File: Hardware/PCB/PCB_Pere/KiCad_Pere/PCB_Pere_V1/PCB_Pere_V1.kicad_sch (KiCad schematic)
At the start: 23 parts, among them CN3 B4B-PH-K-S, U3 Buck LMR51625, U5 Buck LMR51625

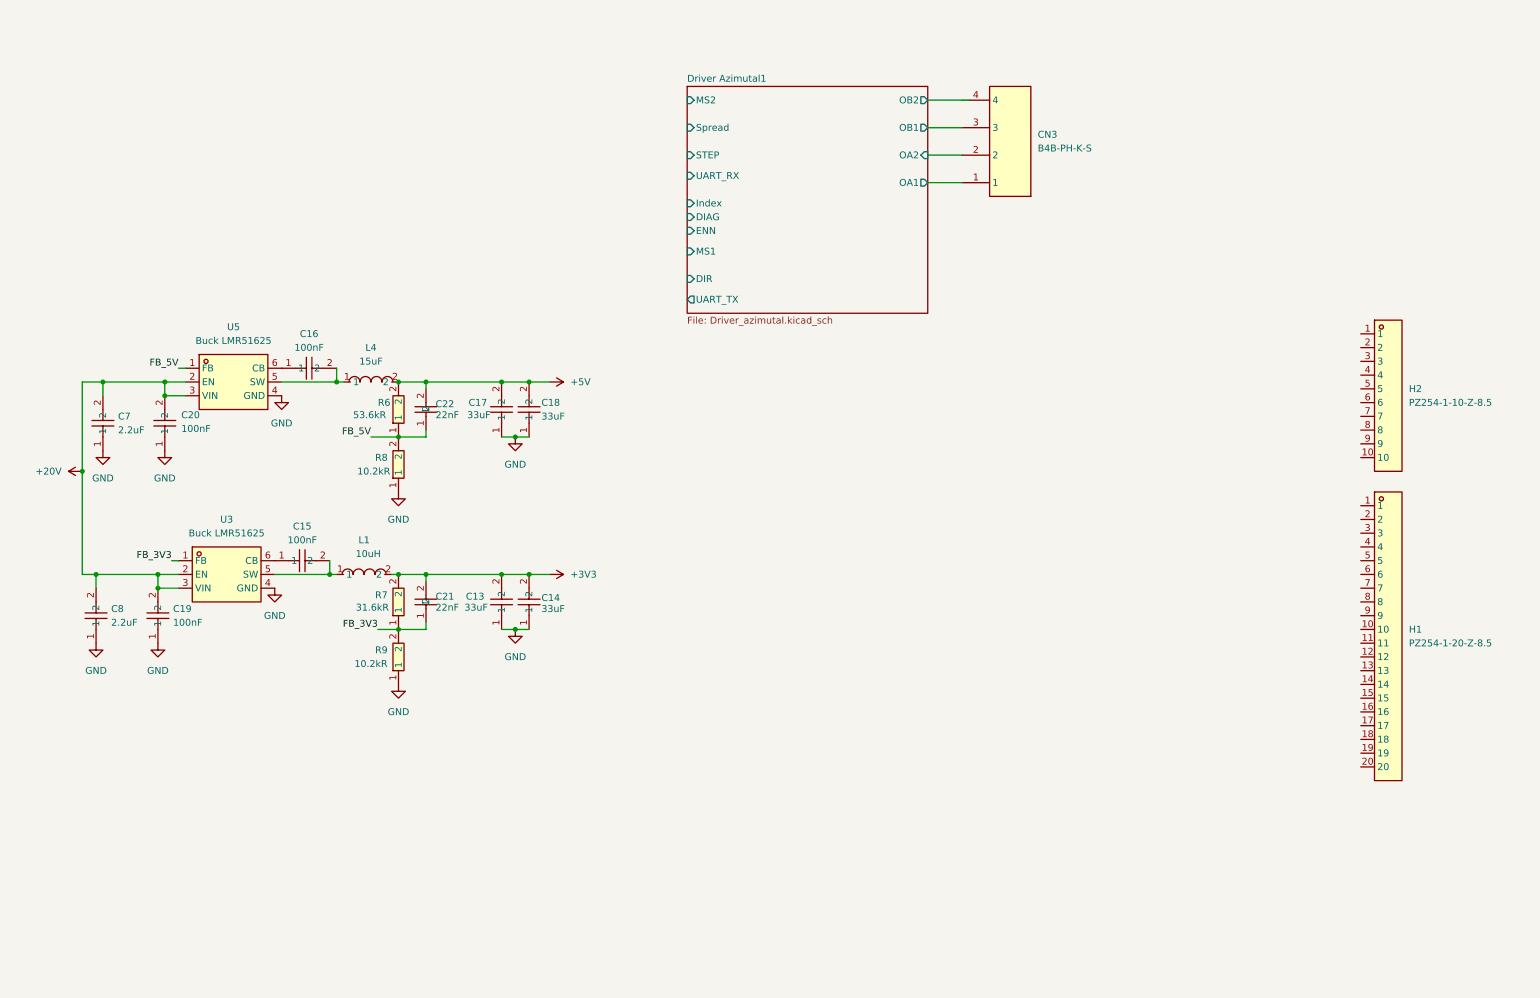
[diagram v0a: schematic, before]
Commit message: Routage toujours en attente oui je sais ça prend 10 000  ans mais it is what is
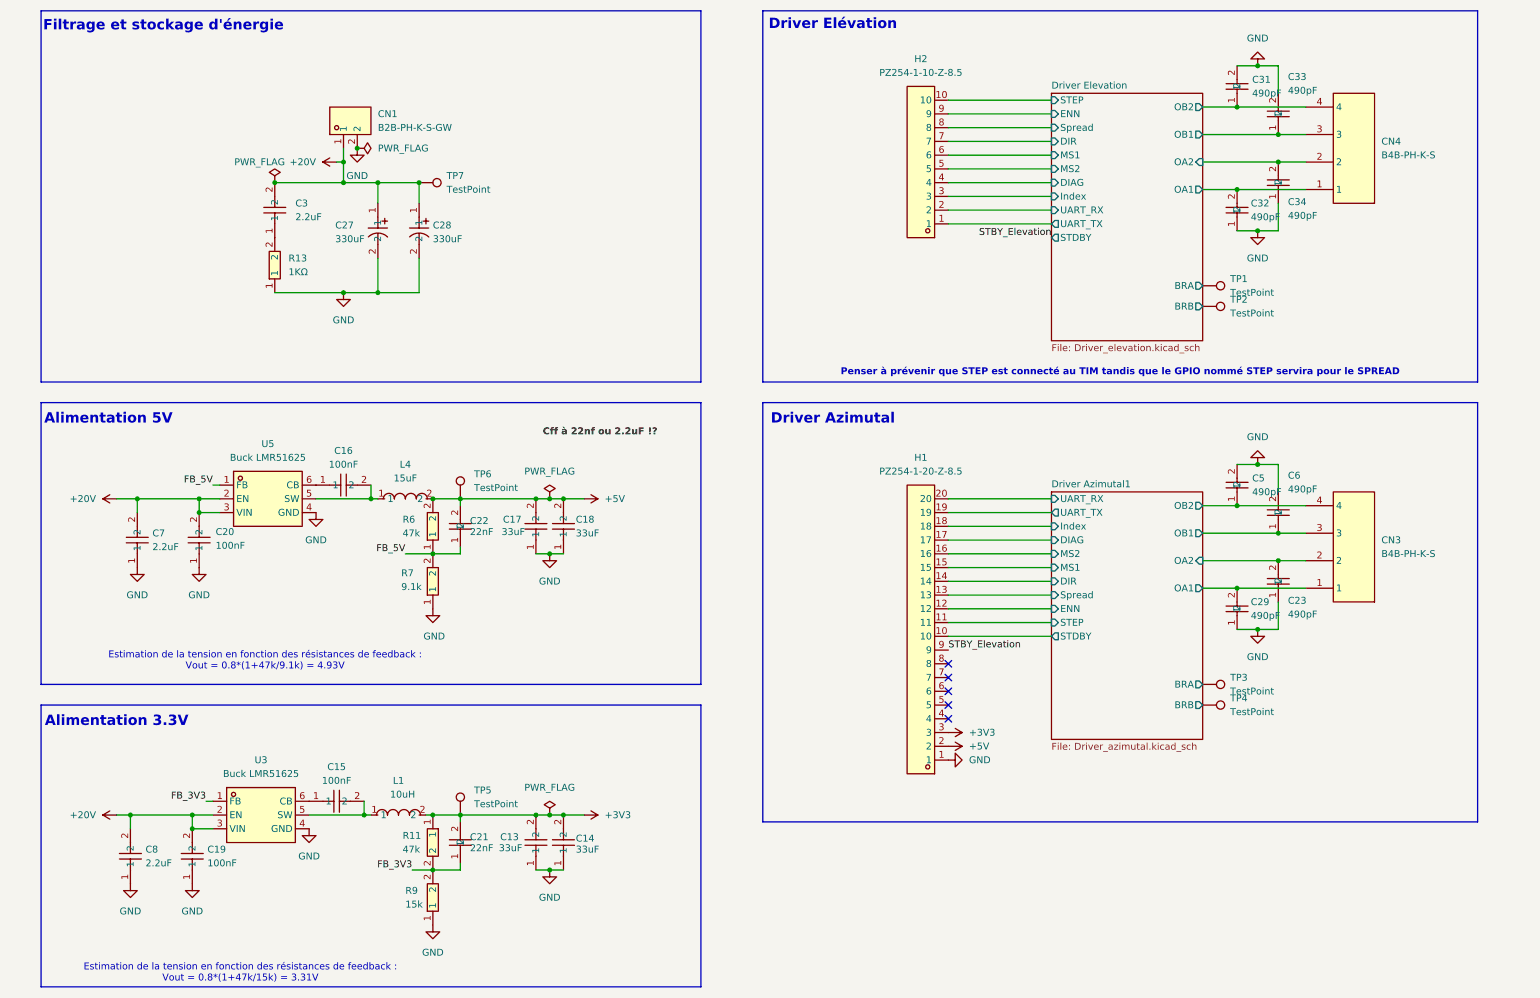
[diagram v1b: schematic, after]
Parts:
- removed R6: 53.6kR, EasyEDA:R0603, symbol EasyEDA:ARG03FTC5362
- removed R7: 31.6kR, EasyEDA:R0603, symbol EasyEDA:ARG03FTC3162
- removed R8, R9: 10.2kR, EasyEDA:R0603, symbol EasyEDA:ARG03FTC10R2
- added C23, C29, C31, C32, C33, C34, C5, C6: 490pF, EasyEDA:C0603, symbol EasyEDA:0603B471K500NT
- added C27, C28: 330uF, EasyEDA:CAP-SMD_BD10.0-L10.3-W10.3-LS11.0-FD, symbol EasyEDA:RVT1H331M1010
- added C3: 2.2uF, EasyEDA:C1206, symbol EasyEDA:TCC1206X7R225K500FT
- added CN1: B2B-PH-K-S-GW, EasyEDA:CONN-TH_B2B-PH-K-S, symbol EasyEDA:B2B-PH-K-S-GW
- added CN4: B4B-PH-K-S, EasyEDA:CONN-TH_B4B-PH-K-S, symbol EasyEDA:B4B-PH-K-S
- added R11, R6: 47k, EasyEDA:R0603, symbol EasyEDA:0603WAF4702T5E
- added R13: 1KΩ, EasyEDA:R0603, symbol EasyEDA:0603WAF1001T5E
- added R7: 9.1k, EasyEDA:R0603, symbol EasyEDA:0603WAF9101T5E
- added R9: 15k, EasyEDA:R0603, symbol EasyEDA:0603WAF1502T5E
- added TP1, TP2, TP3, TP4, TP5: TestPoint, TestPoint:TestPoint_Pad_D2.5mm, symbol Connector:TestPoint
- added TP6, TP7: TestPoint, TestPoint:TestPoint_Pad_2.5x2.5mm, symbol Connector:TestPoint
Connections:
- net +20V: now also C27.1, C28.1, C3.2, CN1.1, TP7.1
- net +3V3: now also H1.3, R11.1, TP5.1
- net +5V: now also H1.2, R6.2, TP6.1
- net Driver Azimutal1/DIAG: now also H1.17
- net Driver Azimutal1/DIR: now also H1.14
- net Driver Azimutal1/ENN: now also H1.12
- net Driver Azimutal1/Index: now also H1.18
- net Driver Azimutal1/MS1: now also H1.15
- net Driver Azimutal1/MS2: now also H1.16
- net Driver Azimutal1/OA1: now also C29.2
- net Driver Azimutal1/OA2: now also C23.2
- net Driver Azimutal1/OB1: now also C6.1
- net Driver Azimutal1/OB2: now also CN3.4, C5.1
- net Driver Azimutal1/STEP: now also H1.11
- net Driver Azimutal1/Spread: now also H1.13
- net Driver Azimutal1/UART_RX: now also H1.20
- net Driver Azimutal1/UART_TX: now also H1.19
- net FB_3V3: now also R11.2, R9.2
- net FB_5V: now also R6.1, R7.2
- net GND: now also H1.1, C23.1, C27.2, C28.2, C29.1, C31.2, C32.1, C33.2, C34.1, C5.2, C6.2, CN1.2, R13.1, R7.1, R9.1
- net Driver Azimutal1/STDBY: now reaches H1.10
- net STBY_Elevation: now reaches H1.9
- net Driver Elevation/UART_TX: now reaches H2.1
- net Driver Elevation/STEP: now reaches H2.10
- net Driver Elevation/UART_RX: now reaches H2.2
- net Driver Elevation/Index: now reaches H2.3
- net Driver Elevation/DIAG: now reaches H2.4
- net Driver Elevation/MS2: now reaches H2.5
- net Driver Elevation/MS1: now reaches H2.6
- net Driver Elevation/DIR: now reaches H2.7
- net Driver Elevation/Spread: now reaches H2.8
- net Driver Elevation/ENN: now reaches H2.9
- new net: C3.1, R13.2
- new net Driver Azimutal1/BRA: TP3.1
- new net Driver Azimutal1/BRB: TP4.1
- new net Driver Elevation/BRA: TP1.1
- new net Driver Elevation/BRB: TP2.1
- new net Driver Elevation/OA1: C32.2, CN4.1
- new net Driver Elevation/OA2: C34.2, CN4.2
- new net Driver Elevation/OB1: C33.1, CN4.3
- new net Driver Elevation/OB2: C31.1, CN4.4
- no-connect marks 0 -> 5
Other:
- added sheet Driver Elevation (Driver_elevation.kicad_sch)
- sheet Driver Azimutal1 ports: added BRA, BRB, STDBY; removed none
- note added: "Alimentation 3.3V"
- note added: "Alimentation 5V"
- note added: "Driver Azimutal"
- note added: "Driver Elévation"
- note added: "Estimation de la tension en fonction des résistances de feedback : Vout = 0.8*(1+47k/15k) = 3.31V"
- note added: "Estimation de la tension en fonction des résistances de feedback : Vout = 0.8*(1+47k/9.1k) = 4.93V"
- note added: "Filtrage et stockage d'énergie"
- note added: "Penser à prévenir que STEP est connecté au TIM tandis que le GPIO nommé STEP servira pour le SPREAD"
- moved on the sheet: C13, C14, C15, C16, C17, C18, C19, C20, C21, C22, C7, C8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
